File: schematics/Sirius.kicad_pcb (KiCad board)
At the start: 2 copper layers, 13 parts, among them J1 DE9_Plug, U1 W65C02SxP, U10 MAX232, U2 W65C51NxP, U3 2764, U4 74LS138, U5 74LS138, X1 TFT680, X2 TFT680

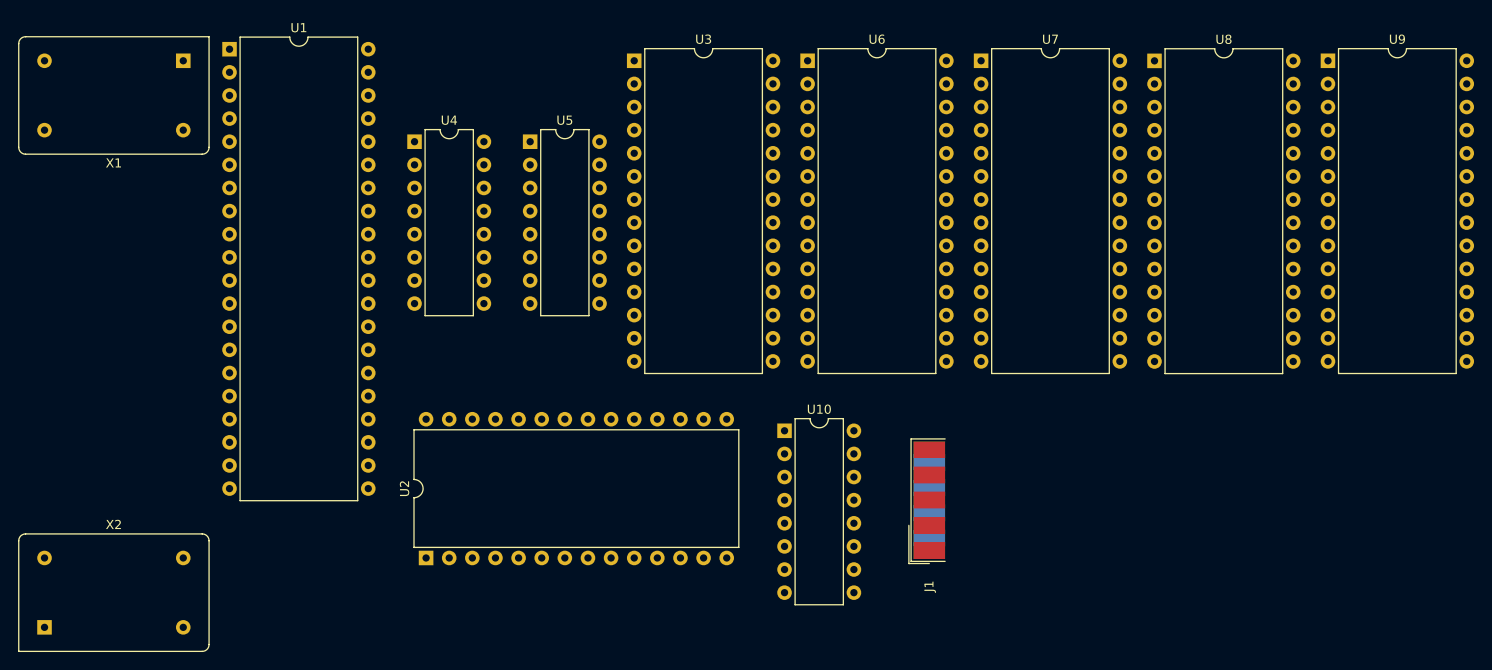
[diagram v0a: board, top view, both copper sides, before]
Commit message: Minor tweaks to signals and PCB layout.
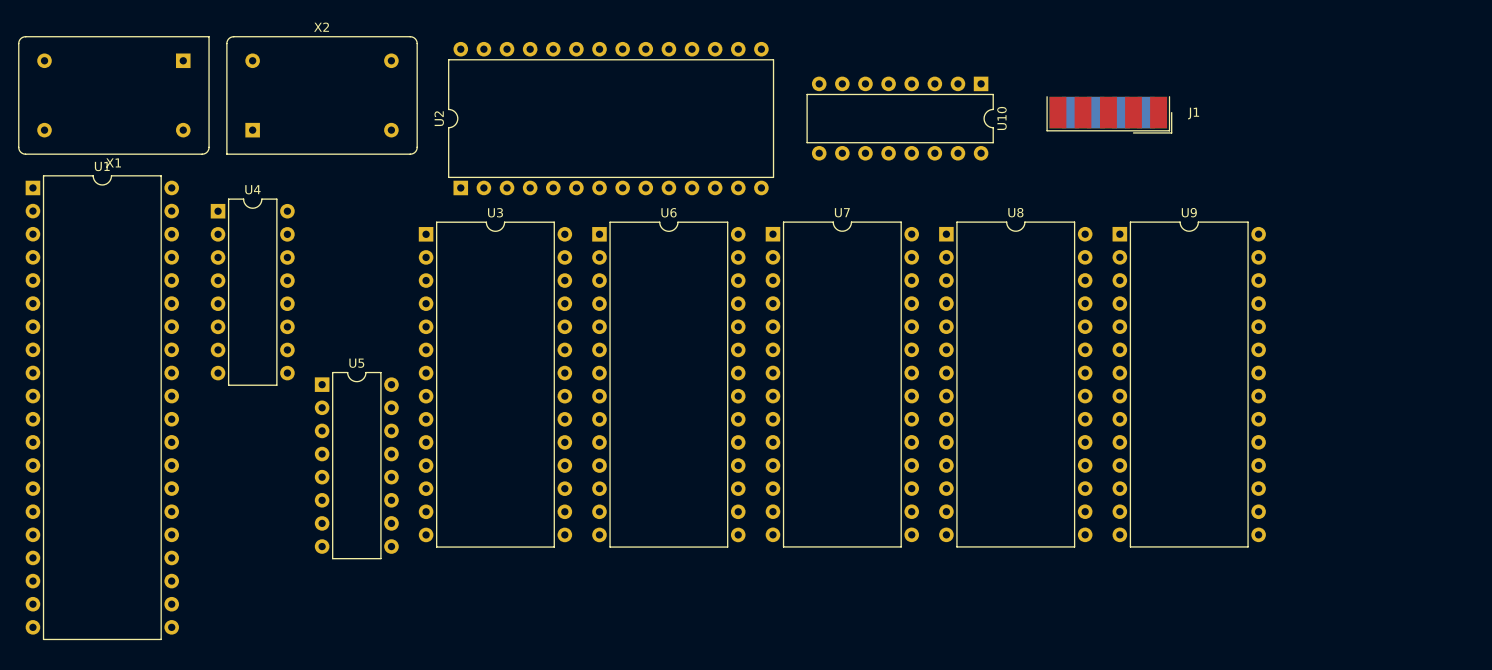
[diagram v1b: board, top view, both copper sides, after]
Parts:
- moved X2 59.2 mm to (38.1, 24.1)
- moved J1 46.9 mm to (132.1, 22.2), turned to 180 degrees
- moved U10 43.8 mm to (118.1, 19.1), turned to -90 degrees
- moved U2 40.8 mm to (61.0, 30.5)
- moved U5 35.1 mm to (45.7, 52.1)
- moved U6 29.8 mm to (76.2, 35.6)
- moved U3 29.8 mm to (57.1, 35.6)
- moved U9 29.8 mm to (133.3, 35.6)
- moved U7 29.8 mm to (95.2, 35.6)
- moved U8 29.7 mm to (114.3, 35.6)
- moved U1 26.4 mm to (14.0, 30.5)
- moved U4 22.9 mm to (34.3, 33.0)
